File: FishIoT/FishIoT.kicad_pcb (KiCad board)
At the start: 4 copper layers, 76.2 x 56.2 mm, 124 parts, among them IC1 RV-3032-C7_32.768KHZ-2.5PPM-T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, J1 VDD_JUMPER, J10 RM_UART, J11 Current Measurement, J13 UART_DEBUG, J2 0705430001, J3 SF72S006VBDR2500, J4 SHF-105-01-L-D-SM, J5 10119313-302TLF, J8 BM05B-ZESS-TBT, J9 Conn_Coaxial, SW1 PTS645SM43SMTR92 LF, SW2 PTS645SM43SMTR92 LF, SW3 PTS645SM43SMTR92 LF, U1 NRF9160-SICA, U10 RM126x, U2 SKY65943-11, U3 TPD3F303DPVR, U4 TPS63000, U5 USBLC6-2P6, U6 CP2102N-Axx-xQFN20, U7 NX3020NAKV, U8 NX3020NAKV, U9 MAX3471

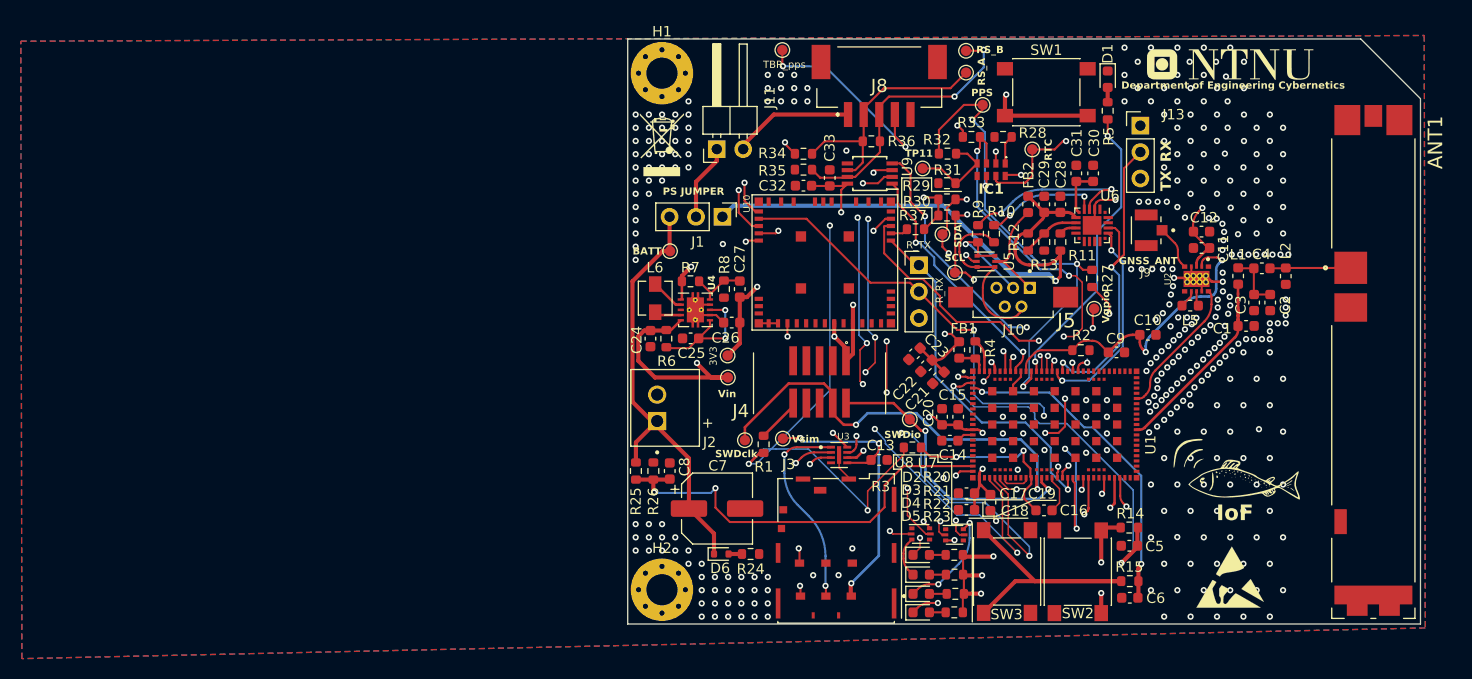
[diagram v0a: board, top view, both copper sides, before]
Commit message: updated schematic and pcb
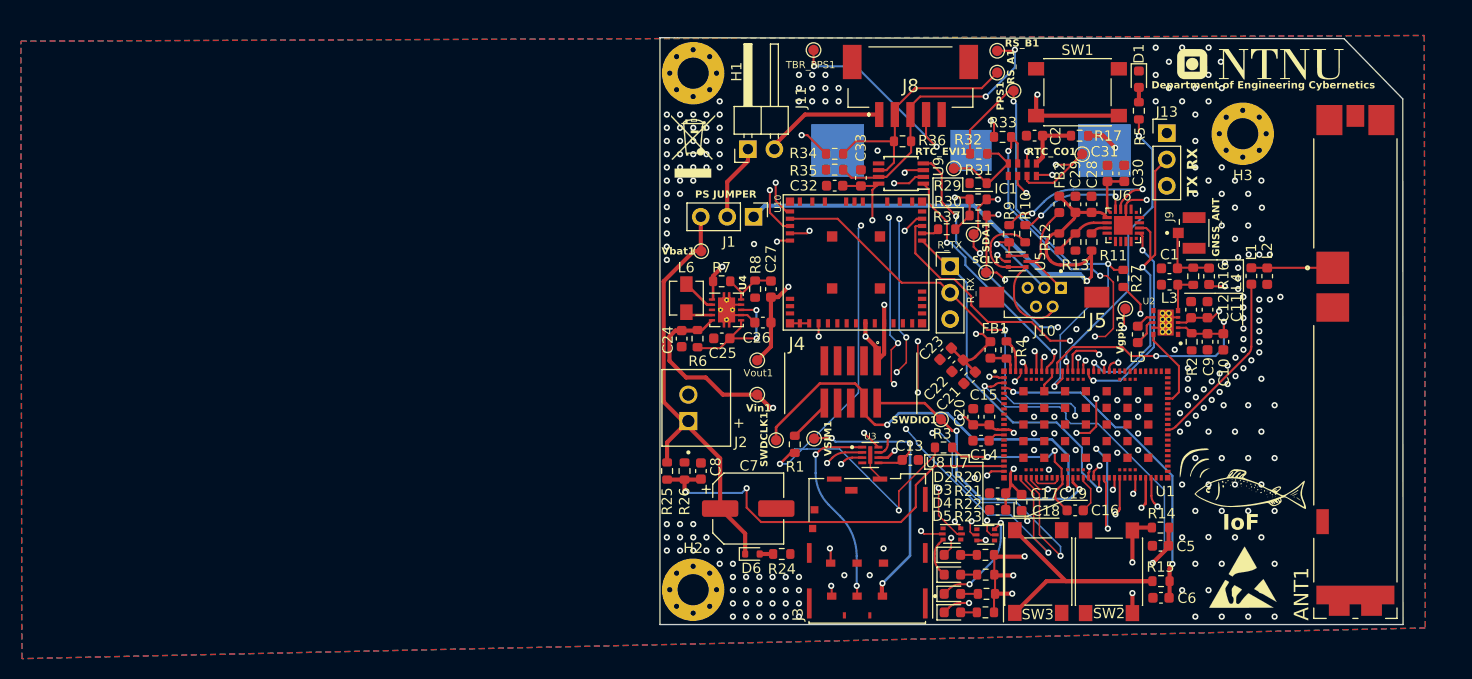
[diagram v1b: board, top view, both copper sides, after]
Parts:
- removed C3: N.C., Capacitor_SMD:C_0603_1608Metric
- removed C4: 3.5pF, Capacitor_SMD:C_0603_1608Metric
- removed R28: 10k, Resistor_SMD:R_0603_1608Metric
- added BT1: 3002, FishIoT_Footprint_library:BAT_3002, B.Cu at (197.3, 67.0)
- added G***: LOGO, FishIoT_Footprint_library:ntnulogoLARGE, B.Cu at (202.4, 98.8)
- added H3: MountingHole_Pad, MountingHole:MountingHole_3mm_Pad_Via, F.Cu at (223.5, 65.3)
- added L3: L, Inductor_SMD:L_0603_1608Metric, F.Cu at (216.4, 79.9)
- added L4: 33nH, Inductor_SMD:L_0603_1608Metric, F.Cu at (220.2, 79.0)
- added R16: R, Resistor_SMD:R_0603_1608Metric, F.Cu at (218.7, 79.0)
- added R17: 120, Resistor_SMD:R_0603_1608Metric, F.Cu at (207.8, 65.5)
- C1: value N.C. -> C
- C2: value N.C. -> 100n
- C33: value 100n -> 0.1u
- R5: value 180 -> 120
- RTC_EVI1: renamed from TP11; value TestPoint -> RTC_EVI
- moved C2 27.8 mm to (203.4, 65.5), turned to 0 degrees
- moved R2 10.7 mm to (218.5, 85.3), turned to 90 degrees
- moved C1 9.22 mm to (216.4, 78.3), turned to 180 degrees
- moved C9 8.81 mm to (220.1, 85.3), turned to -90 degrees
- moved C12 7.57 mm to (218.5, 82.3), turned to 90 degrees
- moved C10 7.28 mm to (221.6, 85.3), turned to 90 degrees
- moved C11 5.96 mm to (220.1, 82.3), turned to -90 degrees
- moved L5 5.75 mm to (213.4, 84.6), turned to 90 degrees
- moved U2 5.13 mm to (216.0, 83.5), turned to 180 degrees
- moved RTC_CO1 4.82 mm to (208.0, 67.3)
- moved J9 4.62 mm to (218.8, 74.9), turned to -90 degrees
- moved Vin1 3.27 mm to (176.8, 90.4)
- moved PPS1 3.26 mm to (201.4, 61.2)
- moved REF** 3.00 mm to (170.6, 66.5)
- moved J10 3.00 mm to (195.3, 78.1)
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- renumbered PPS to PPS1, RS_A to RS_A1, RS_B to RS_B1, RTC to RTC_CO1, SCL to SCL1, SDA to SDA1, SWDclk to SWDCLK1, SWDio to SWDIO1, TBR_pps to TBR_PPS1, Vsim to VSIM1, BATT to Vbat1, Vgpio to Vgpio1, Vin to Vin1, 3V3 to Vout1
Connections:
- C1 pad 1: /LTE_RF1 -> Net-(J9-In)
- C2 pad 1: Net-(C2-Pad1) -> GND
- C2 pad 2: GND -> Net-(IC1-VBACKUP)
- H1 pad 1: unconnected-(H1-Pad1) -> GND
- H2 pad 1: unconnected-(H2-Pad1) -> GND
- J9 pad 1: /GPS_RF_ANT -> Net-(J9-In)
- L1 pad 2: Net-(C2-Pad1) -> Net-(ANT1-FEED)
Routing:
- net Net-(J9-In): track 0.00 -> 6.51 mm
- net Net-(C2-Pad1): track 5.60 -> 0.00 mm
- net /GPS_RF1: track 13.4 -> 7.90 mm
- net /VREG_IN: track 60.0 -> 64.9 mm
- net /GPS_EN: track 31.0 -> 26.5 mm
- net Net-(BT1-PadP1): track 0.00 -> 3.08 mm, vias 0 -> 1
- net +3V3: track 80.6 -> 83.5 mm, vias 20 -> 21
- net Net-(IC1-VBACKUP): track 2.81 -> 5.53 mm
- net GND: track 41.0 -> 38.9 mm, vias 338 -> 224
- net Net-(U2-AMP_IN): track 1.43 -> 2.75 mm
- net /RTC_CLOCKOUT: track 36.7 -> 35.6 mm
- net /PPS: track 47.1 -> 48.0 mm
- net /nRF_UART_RX: track 32.8 -> 31.9 mm
- net /nRF_UART_TX: track 27.9 -> 27.0 mm
- net /LTE_RF1: track 18.3 -> 17.5 mm
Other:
- board size 76.2 x 56.2 mm -> 71.4 x 56.4 mm
